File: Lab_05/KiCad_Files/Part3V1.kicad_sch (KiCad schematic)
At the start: 29 parts, among them Q1 NPN, Q2 PNP, Q3 NPN, Q4 NPN, Q5 NPN, Q6 NPN, Q7 NPN, Q8 NPN, Q9 PNP

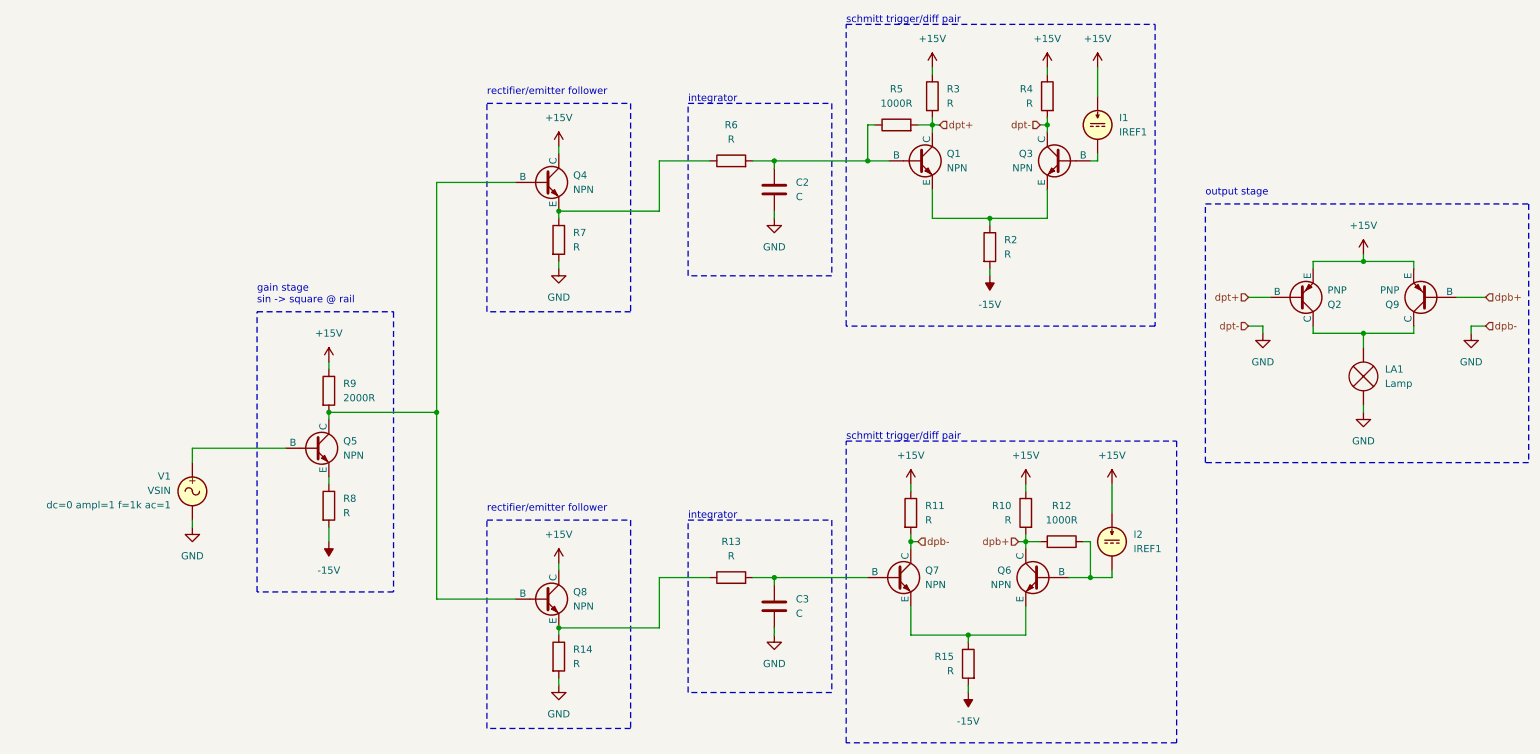
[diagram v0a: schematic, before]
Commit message: Continue Lab 5
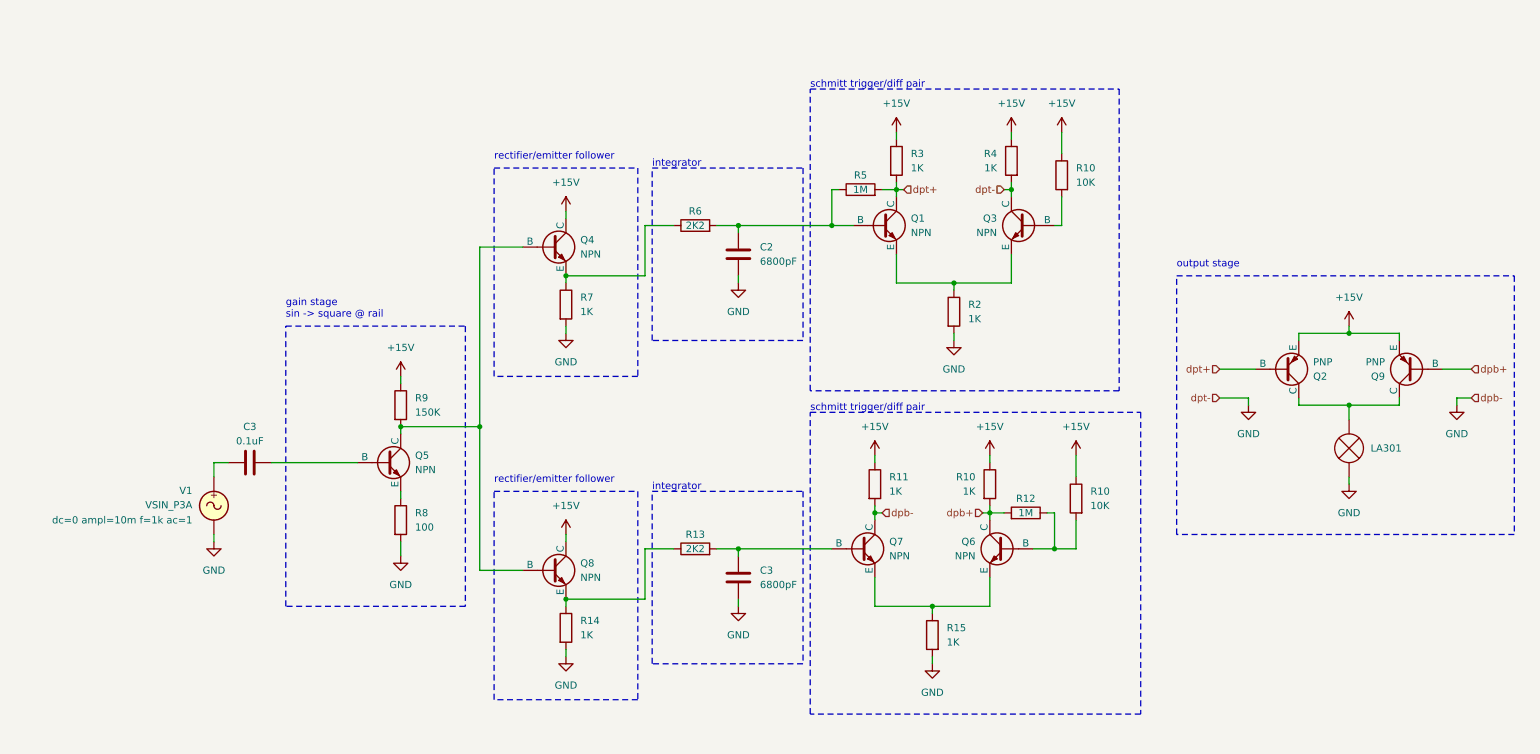
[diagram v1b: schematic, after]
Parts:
- removed I1, I2: IREF1, symbol Simulation_SPICE:IDC
- removed LA1: Lamp, symbol Device:Lamp
- added C3: 0.1uF, symbol Device:C
- added LA301: ${SIM.PARAMS}, symbol Device:Lamp
- added R10 (x2): 10K, symbol Device:R
- C2, C3: value C -> 6800pF
- R10, R11, R14, R15, R2, R3, R4, R7: value R -> 1K
- R12, R5: value 1000R -> 1M
- R13, R6: value R -> 2K2
- R8: value R -> 100
- R9: value 2000R -> 150K
- V1: value VSIN -> VSIN_P3A
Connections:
- net -15V is gone; now on net GND: R15.2, R2.2, R8.2
- net +15V: now also R10.1, R10.1
- net GND: now also LA301.1 (-)
- net at Q2.1 (C), Q9.1 (C): now also LA301.2 (+)
- net at Q6.2 (B), R12.1: now also R10.2
- net at Q3.2 (B): now also R10.2
- net at V1.1: now also C3.1; no longer Q5.2 (B)
- new net: C3.2, Q5.2 (B)
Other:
- company: (none) -> Jim Horwitz & Mark Vaughn, Jork Incorporated
- moved on the sheet: C2, C3, Q1, Q2, Q3, Q4, Q5, Q6, Q7, Q8, Q9, R10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
